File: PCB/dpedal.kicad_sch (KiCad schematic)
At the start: 19 parts, among them J1 USB_C_Receptacle_USB2.0, SW1 SW_Push, SW2 SW_Push, SW3 SW_Push, SW4 SW_Push, SW5 RESET, SW6 FLASH, U1 STM32F072C8Tx, U2 LDO

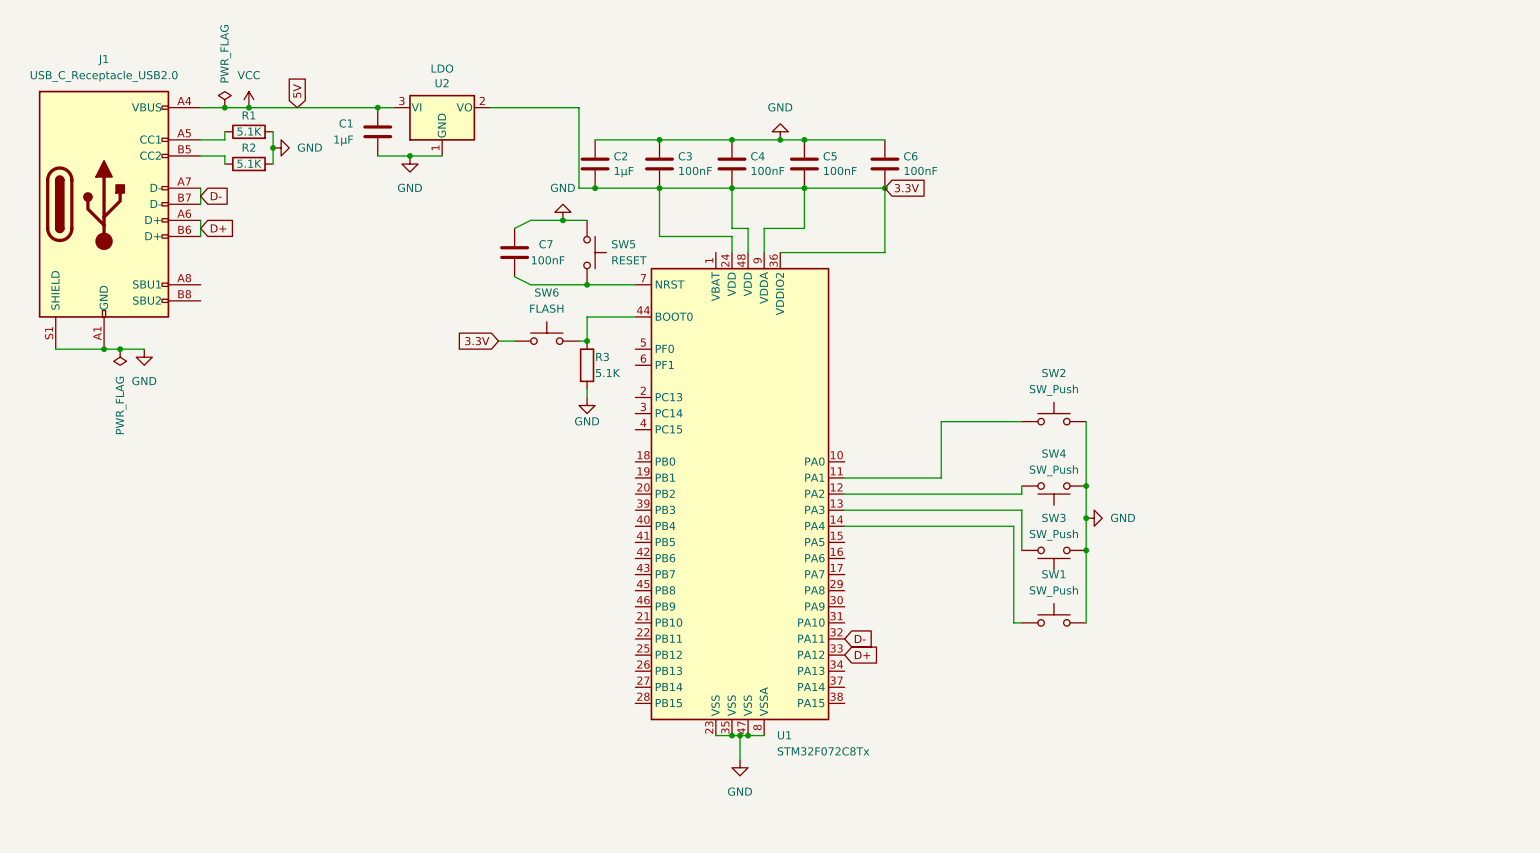
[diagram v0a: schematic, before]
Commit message: PCB v2
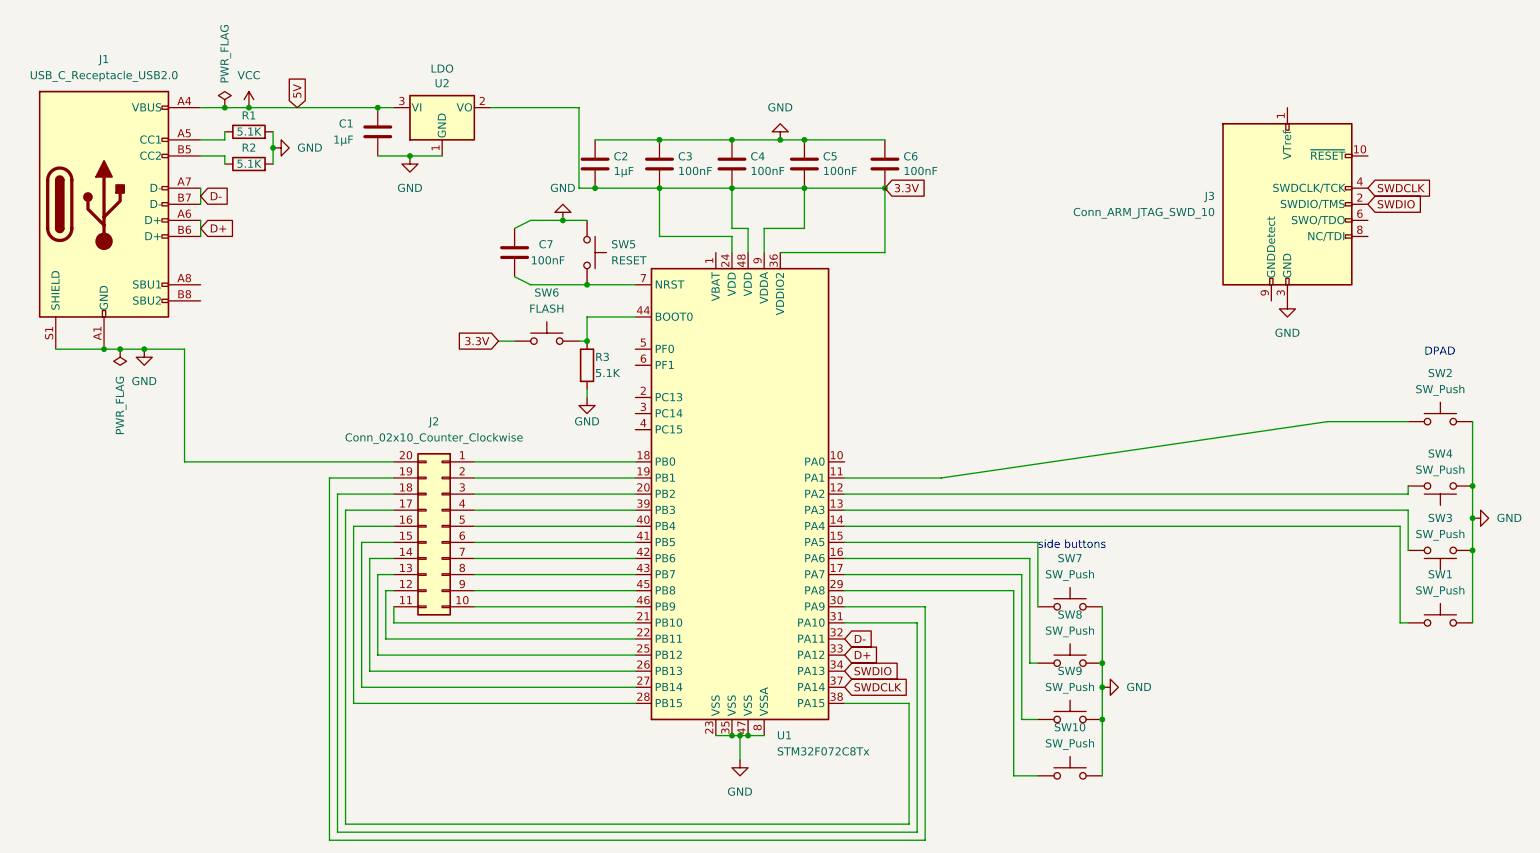
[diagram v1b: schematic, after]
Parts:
- added J2: Conn_02x10_Counter_Clockwise, Connector_IDC:IDC-Header_2x10_P2.54mm_Horizontal, symbol Connector_Generic:Conn_02x10_Counter_Clockwise
- added J3: Conn_ARM_JTAG_SWD_10, Connector_PinHeader_1.27mm:PinHeader_2x05_P1.27mm_Vertical, symbol Connector:Conn_ARM_JTAG_SWD_10
- added SW10, SW7, SW8, SW9: SW_Push, Switch_Keyboard_Hotswap_Kailh:SW_Hotswap_Kailh_MX_plated_1.00u, symbol Switch:SW_Push
- SW1, SW2, SW3, SW4: footprint Button_Switch_Keyboard:SW_Cherry_MX_1.00u_Plate -> Switch_Keyboard_Hotswap_Kailh:SW_Hotswap_Kailh_MX_plated_1.00u
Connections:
- net GND: now also J2.20 (Pin_20), J3.3 (GND), J3.5 (GND), SW10.2, SW7.2, SW8.2, SW9.2
- net at U1.15 (PA5): now also SW7.1
- net at U1.16 (PA6): now also SW8.1
- net at U1.17 (PA7): now also SW9.1
- net at U1.18 (PB0): now also J2.1 (Pin_1)
- net at U1.19 (PB1): now also J2.2 (Pin_2)
- net at U1.20 (PB2): now also J2.3 (Pin_3)
- net at U1.21 (PB10): now also J2.11 (Pin_11)
- net at U1.22 (PB11): now also J2.12 (Pin_12)
- net at U1.25 (PB12): now also J2.13 (Pin_13)
- net at U1.26 (PB13): now also J2.14 (Pin_14)
- net at U1.27 (PB14): now also J2.15 (Pin_15)
- net at U1.28 (PB15): now also J2.16 (Pin_16)
- net at U1.29 (PA8): now also SW10.1
- net at U1.30 (PA9): now also J2.19 (Pin_19)
- net at U1.31 (PA10): now also J2.18 (Pin_18)
- net SWDIO: now reaches U1.34 (PA13)
- net SWDIO: now also J3.2 (SWDIO/TMS)
- net SWDCLK: now reaches U1.37 (PA14)
- net SWDCLK: now also J3.4 (SWDCLK/TCK)
- net at U1.38 (PA15): now also J2.17 (Pin_17)
- net at U1.39 (PB3): now also J2.4 (Pin_4)
- net at U1.40 (PB4): now also J2.5 (Pin_5)
- net at U1.41 (PB5): now also J2.6 (Pin_6)
- net at U1.42 (PB6): now also J2.7 (Pin_7)
- net at U1.43 (PB7): now also J2.8 (Pin_8)
- net at U1.45 (PB8): now also J2.9 (Pin_9)
- net at U1.46 (PB9): now also J2.10 (Pin_10)
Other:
- note added: "DPAD"
- note added: "side buttons"
- moved on the sheet: SW1, SW2, SW3, SW4

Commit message: PCB v2 More
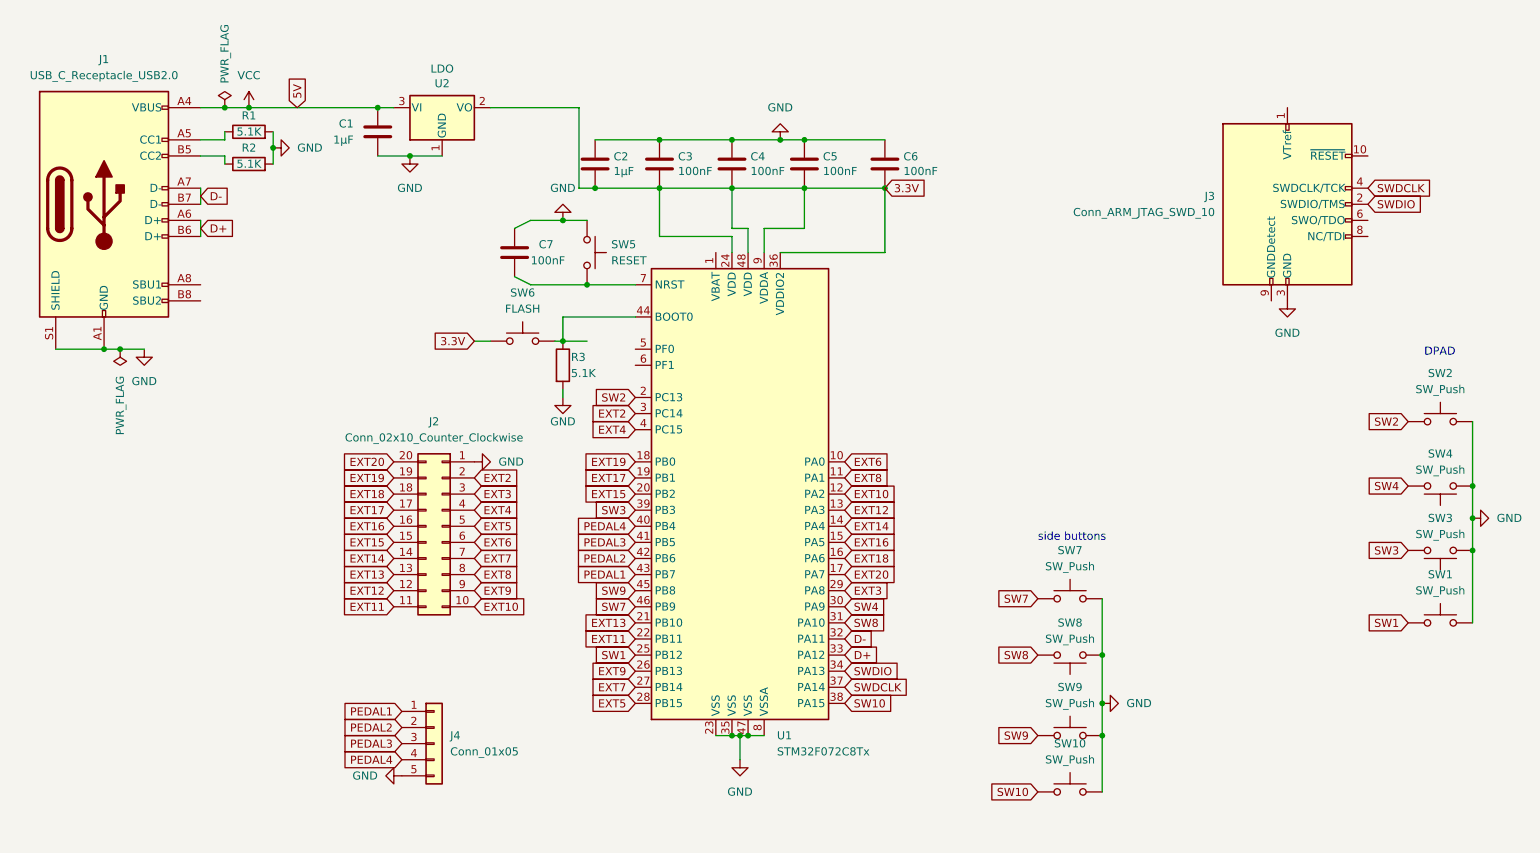
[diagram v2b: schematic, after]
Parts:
- added J4: Conn_01x05, Connector_PinHeader_1.00mm:PinHeader_1x05_P1.00mm_Horizontal, symbol Connector_Generic:Conn_01x05
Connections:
- net GND: now also J2.1 (Pin_1), SW8.1, J4.5 (Pin_5); no longer J2.20 (Pin_20), SW8.2
- net EXT10: now reaches U1.12 (PA2)
- net EXT10: now also J2.10 (Pin_10); no longer SW4.2
- net EXT3: now reaches U1.29 (PA8)
- net EXT3: now also J2.3 (Pin_3); no longer SW10.1
- net EXT18: now reaches U1.16 (PA6)
- net EXT18: now also J2.18 (Pin_18); no longer SW8.1
- net EXT19: now reaches U1.18 (PB0)
- net EXT19: now also J2.19 (Pin_19); no longer J2.1 (Pin_1)
- net SW7: now reaches U1.46 (PB9)
- net SW7: now also SW7.1; no longer J2.10 (Pin_10)
- net EXT11: now reaches J2.11 (Pin_11)
- net EXT11: now also U1.22 (PB11); no longer U1.21 (PB10)
- net EXT12: now reaches J2.12 (Pin_12)
- net EXT12: now also U1.13 (PA3); no longer U1.22 (PB11)
- net EXT13: now reaches J2.13 (Pin_13)
- net EXT13: now also U1.21 (PB10); no longer U1.25 (PB12)
- net EXT14: now reaches J2.14 (Pin_14)
- net EXT14: now also U1.14 (PA4); no longer U1.26 (PB13)
- net EXT15: now reaches J2.15 (Pin_15)
- net EXT15: now also U1.20 (PB2); no longer U1.27 (PB14)
- net EXT16: now reaches J2.16 (Pin_16)
- net EXT16: now also U1.15 (PA5); no longer U1.28 (PB15)
- net EXT17: now reaches J2.17 (Pin_17)
- net EXT17: now also U1.19 (PB1); no longer U1.38 (PA15)
- net SW8: now reaches U1.31 (PA10)
- net SW8: now also SW8.2; no longer J2.18 (Pin_18)
- net SW4: now reaches U1.30 (PA9)
- net SW4: now also SW4.2; no longer J2.19 (Pin_19)
- net EXT2: now reaches J2.2 (Pin_2)
- net EXT2: now also U1.3 (PC14); no longer U1.19 (PB1)
- net EXT4: now reaches J2.4 (Pin_4)
- net EXT4: now also U1.4 (PC15); no longer U1.39 (PB3)
- net EXT5: now reaches J2.5 (Pin_5)
- net EXT5: now also U1.28 (PB15); no longer U1.40 (PB4)
- net EXT6: now reaches J2.6 (Pin_6)
- net EXT6: now also U1.10 (PA0); no longer U1.41 (PB5)
- net EXT7: now reaches J2.7 (Pin_7)
- net EXT7: now also U1.27 (PB14); no longer U1.42 (PB6)
- net EXT8: now reaches J2.8 (Pin_8)
- net EXT8: now also U1.11 (PA1); no longer U1.43 (PB7)
- net EXT9: now reaches J2.9 (Pin_9)
- net EXT9: now also U1.26 (PB13); no longer U1.45 (PB8)
- net EXT20: now reaches U1.17 (PA7)
- net EXT20: now also J2.20 (Pin_20); no longer SW9.1
- net SW2: now reaches SW2.1
- net SW2: now also U1.2 (PC13); no longer U1.11 (PA1)
- net SW3: now reaches SW3.2
- net SW3: now also U1.39 (PB3); no longer U1.13 (PA3)
- net SW1: now reaches SW1.1
- net SW1: now also U1.25 (PB12); no longer U1.14 (PA4)
- new net PEDAL1: J4.1 (Pin_1), U1.43 (PB7)
- new net PEDAL2: J4.2 (Pin_2), U1.42 (PB6)
- new net PEDAL3: J4.3 (Pin_3), U1.41 (PB5)
- new net PEDAL4: J4.4 (Pin_4), U1.40 (PB4)
- new net SW10: SW10.1, U1.38 (PA15)
- new net SW9: SW9.1, U1.45 (PB8)
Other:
- moved on the sheet: R3, SW10, SW6, SW7, SW8, SW9
